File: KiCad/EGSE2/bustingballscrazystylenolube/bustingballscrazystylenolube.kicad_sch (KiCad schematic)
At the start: 0 parts

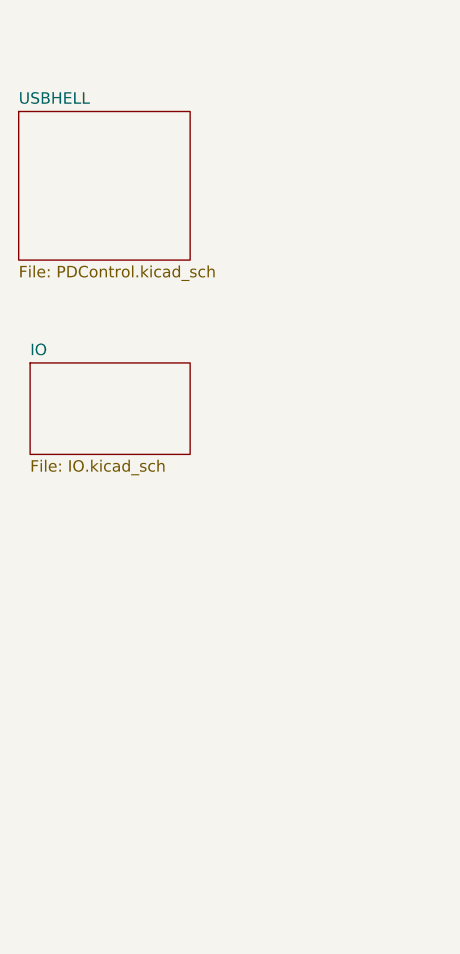
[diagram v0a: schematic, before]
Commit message: here comes the
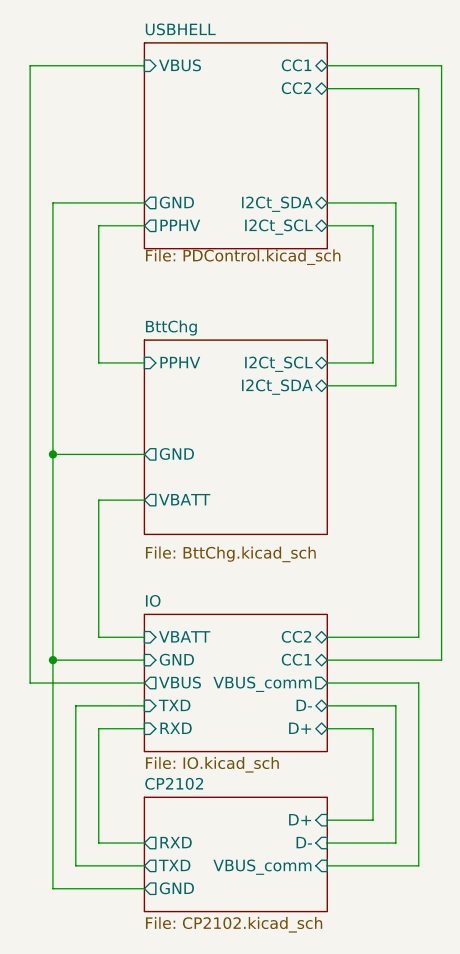
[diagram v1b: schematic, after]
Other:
- added sheet BttChg (BttChg.kicad_sch)
- added sheet CP2102 (CP2102.kicad_sch)
- sheet IO ports: added CC1, CC2, D+, D-, GND, RXD, TXD, VBATT, VBUS, VBUS_comm; removed none
- sheet USBHELL ports: added CC1, CC2, GND, I2Ct_SCL, I2Ct_SDA, PPHV, VBUS; removed none
